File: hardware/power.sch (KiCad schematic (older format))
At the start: 24 parts, among them Q1 Si3129DV, U1 MAX5035BUSA, U2 NCP1117-3.3_SOT223

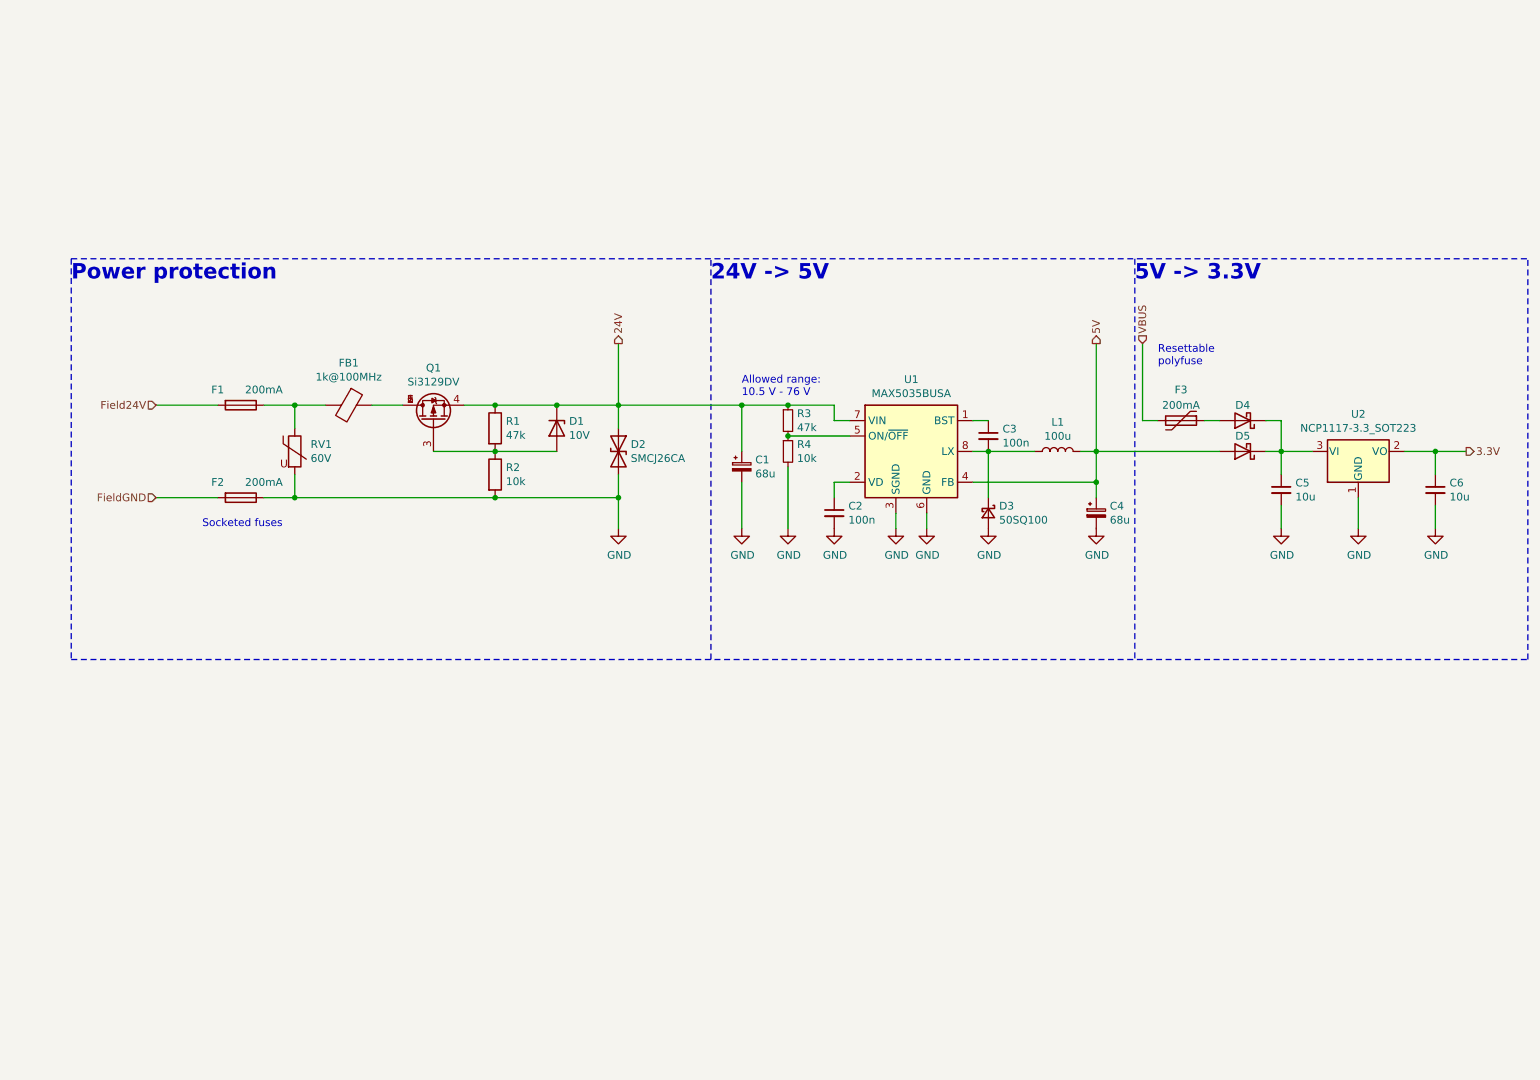
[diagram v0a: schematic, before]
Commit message: Changed power again
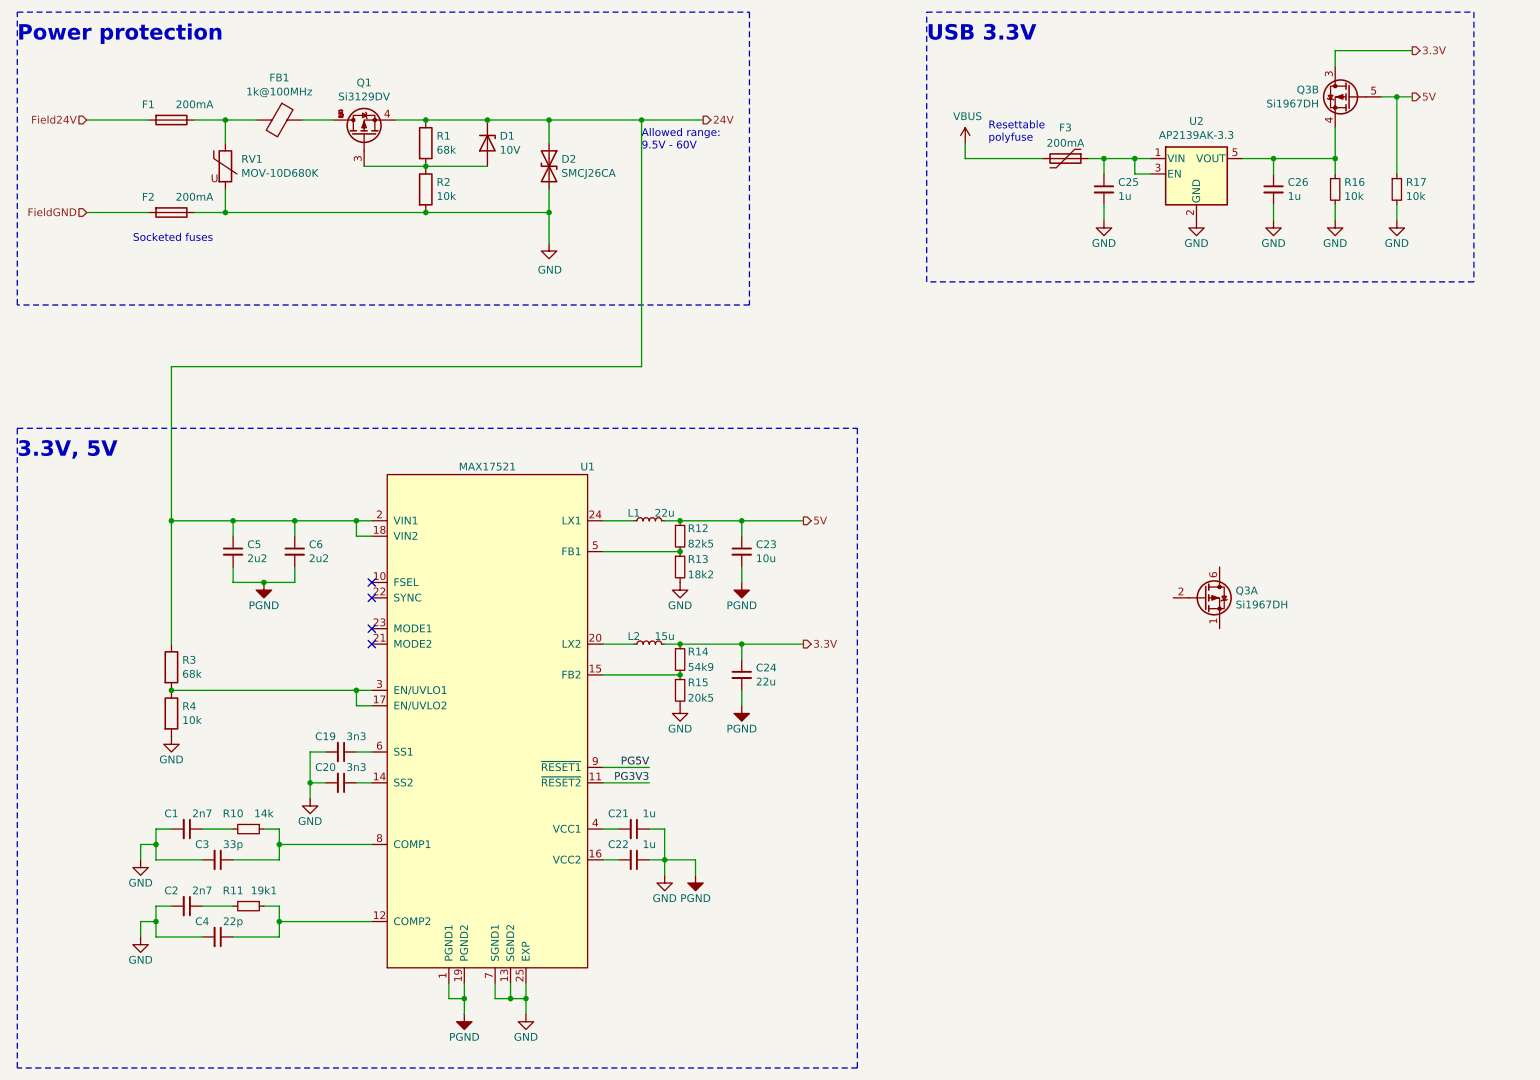
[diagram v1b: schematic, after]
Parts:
- removed C1, C4: 68u, symbol Device:CP_Small
- removed D3: 50SQ100, symbol Device:D_Schottky_Small
- removed D4, D5: D_Schottky, Diode_SMD:D_SMA, symbol Device:D_Schottky
- removed L1: 100u, symbol Device:L
- removed R3: 47k, symbol Device:R_Small
- removed R4: 10k, symbol Device:R_Small
- removed U1: MAX5035BUSA, Package_SO:SOIC-8_3.9x4.9mm_P1.27mm, symbol Regulator_Switching:MAX5035BUSA
- removed U2: NCP1117-3.3_SOT223, Package_TO_SOT_SMD:SOT-223-3_TabPin2, symbol Regulator_Linear:NCP1117-3.3_SOT223
- added C1: 2n7, Capacitor_SMD:C_0805_2012Metric, symbol Device:C_Small
- added C19, C20: 3n3, Capacitor_SMD:C_0805_2012Metric, symbol Device:C_Small
- added C21, C22, C25, C26: 1u, Capacitor_SMD:C_0805_2012Metric, symbol Device:C_Small
- added C23: 10u, Capacitor_SMD:C_0805_2012Metric, symbol Device:C_Small
- added C24: 22u, Capacitor_SMD:C_0805_2012Metric, symbol Device:C_Small
- added C4: 22p, Capacitor_SMD:C_0805_2012Metric, symbol Device:C_Small
- added L1: 22u, symbol Device:L_Small
- added L2: 15u, symbol Device:L_Small
- added Q3: Si1967DH, Package_TO_SOT_SMD:SOT-363_SC-70-6_Handsoldering, symbol Device:Q_DUAL_PMOS_S1G1D2S2G2D1
- added R10: 14k, Resistor_SMD:R_0805_2012Metric, symbol Device:R_Small
- added R11: 19k1, Resistor_SMD:R_0805_2012Metric, symbol Device:R_Small
- added R12: 82k5, Resistor_SMD:R_0805_2012Metric, symbol Device:R_Small
- added R13: 18k2, Resistor_SMD:R_0805_2012Metric, symbol Device:R_Small
- added R14: 54k9, Resistor_SMD:R_0805_2012Metric, symbol Device:R_Small
- added R15: 20k5, Resistor_SMD:R_0805_2012Metric, symbol Device:R_Small
- added R16, R17: 10k, Resistor_SMD:R_0805_2012Metric, symbol Device:R_Small
- added R3: 68k, Resistor_SMD:R_0805_2012Metric, symbol Device:R
- added R4: 10k, Resistor_SMD:R_0805_2012Metric, symbol Device:R
- added U1: MAX17521, MAX17521:QFN50P500X400X80-25N, symbol MAX17521ATG_:MAX17521
- added U2: AP2139AK-3.3, Package_TO_SOT_SMD:SOT-23-5, symbol Regulator_Linear:AP2127K-3.3
- C2: value 100n -> 2n7
- C3: value 100n -> 33p
- C5, C6: value 10u -> 2u2
- FB1: footprint (none) -> Inductor_SMD:L_0805_2012Metric
- R1: value 47k -> 68k; footprint (none) -> Resistor_SMD:R_0805_2012Metric
- R2: footprint (none) -> Resistor_SMD:R_0805_2012Metric
- RV1: value 60V -> MOV-10D680K; footprint (none) -> Varistor:RV_Disc_D12mm_W4.4mm_P7.5mm
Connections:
- net 24V: now also C5.1, C6.1, R3.1, U1.18 (VIN2), U1.2 (VIN1)
- net 3.3V: now also C24.1, L2.2, Q3.3 (D), R14.1; no longer C6.1
- net 5V: now also C23.1, L1.2, Q3.5 (G), R12.1, R17.1
- net GND: now also C3.2, C1.2, C19.2, C20.2, C21.1, C22.1, C23.2, C24.2, C25.2, C26.2, C4.2, R13.2, R15.2, R16.2, R17.2, R4.2, U1.1 (PGND1), U1.13 (SGND2), U1.19 (PGND2), U1.25 (EXP), U1.7 (SGND1), U2.2 (GND)
- net at C3.1: now also R10.1, U1.8 (COMP1)
- net at C2.1: now also R11.2
- net at F3.1: now also C25.1, U2.1 (VIN), U2.3 (EN)
- new net: C4.1, R11.1, U1.12 (COMP2)
- new net: C20.1, U1.14 (SS2)
- new net: R14.2, R15.1, U1.15 (FB2)
- new net: C22.2, U1.16 (VCC2)
- new net: R3.2, R4.1, U1.17 (EN/UVLO2), U1.3 (EN/UVLO1)
- new net: L2.1, U1.20 (LX2)
- new net: L1.1, U1.24 (LX1)
- new net: C21.2, U1.4 (VCC1)
- new net: R12.2, R13.1, U1.5 (FB1)
- new net: C19.1, U1.6 (SS1)
- new net: C1.1, R10.2
- new net: C26.1, Q3.4 (S), R16.1, U2.5 (VOUT)
- new net PG3V3: U1.11 (~RESET2)
- new net PG5V: U1.9 (~RESET1)
- no-connect marks 0 -> 4
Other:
- note added: "3.3V, 5V"
- note added: "Allowed range:\n9.5V - 60V"
- note added: "USB 3.3V"
- note removed: "24V -> 5V"
- note removed: "5V -> 3.3V"
- note removed: "Allowed range:\n10.5 V - 76 V"
- moved on the sheet: D1, D2, F1, F2, F3, FB1, Q1, R1, R2, RV1
